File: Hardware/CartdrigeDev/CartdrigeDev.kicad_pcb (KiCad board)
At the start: 2 copper layers, 80 x 14.5 mm, 2 parts, among them J1 Conn_02x30_Odd_Even, J2 PORT1

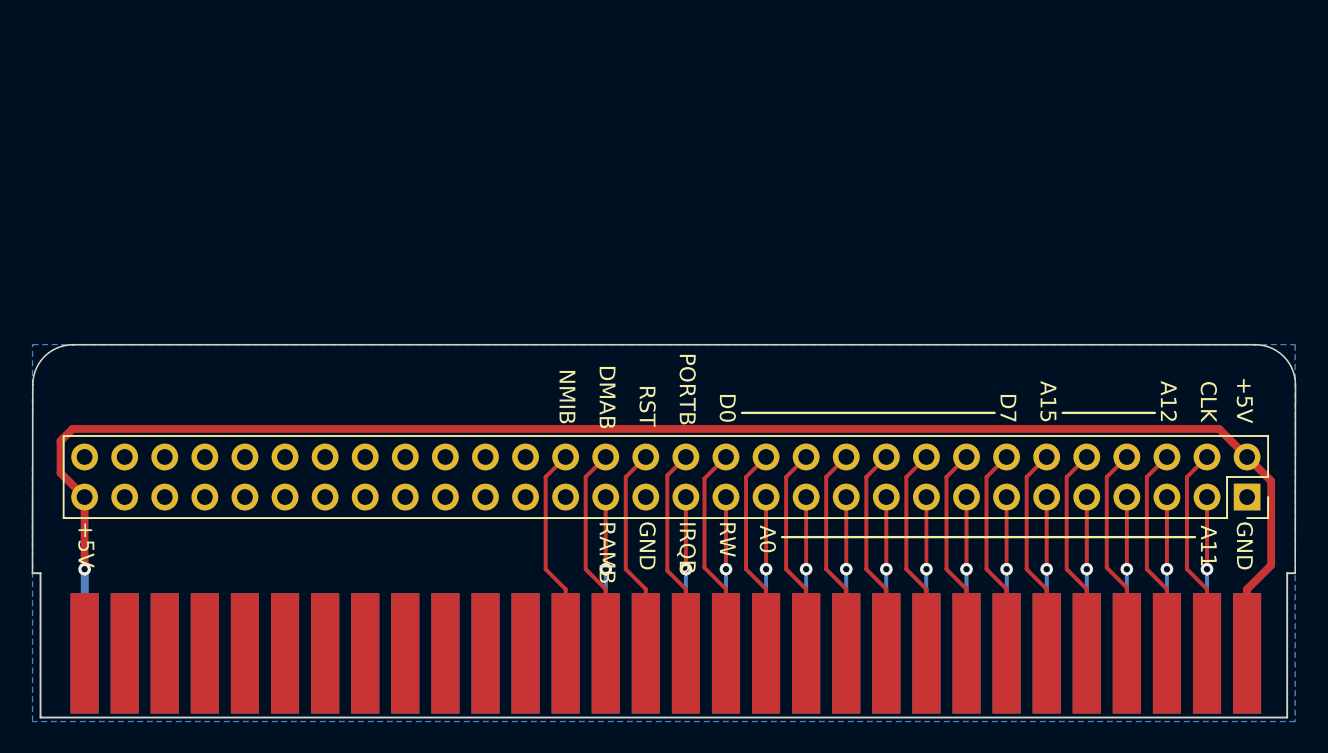
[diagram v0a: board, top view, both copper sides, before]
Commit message: Version 1.3
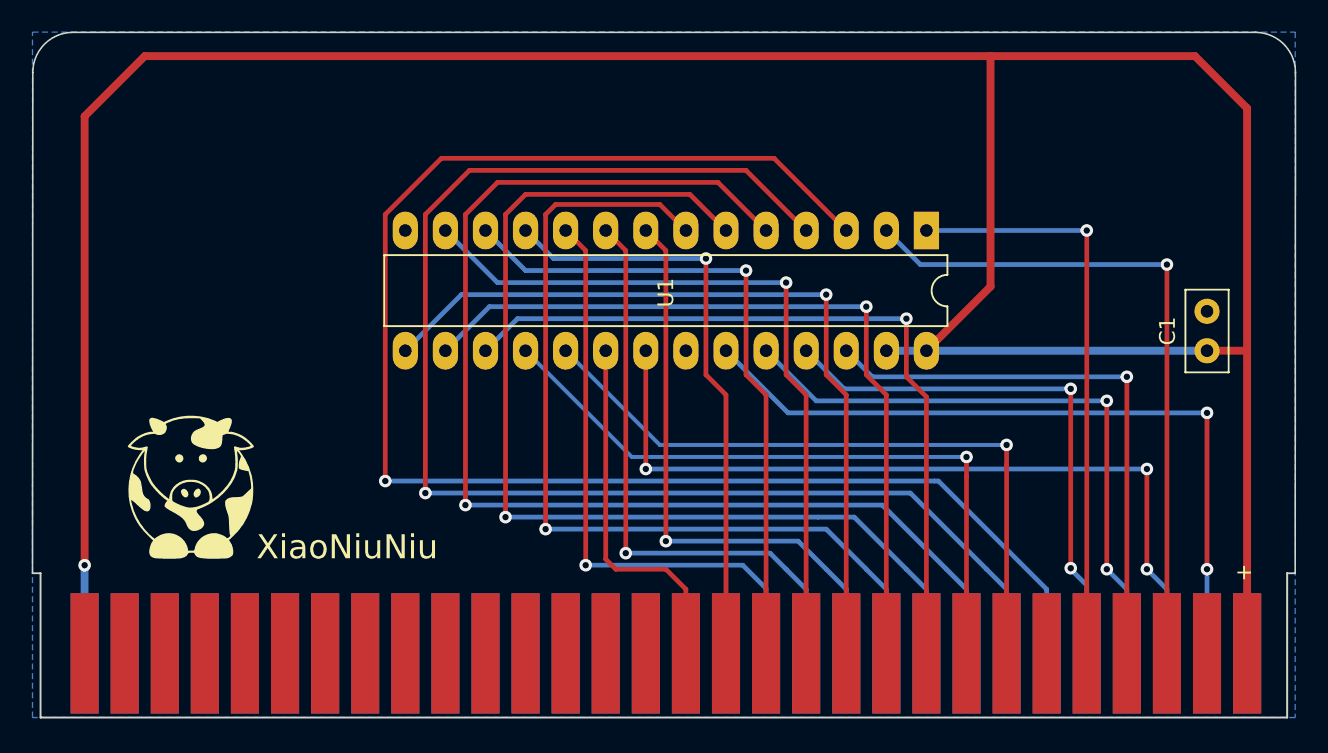
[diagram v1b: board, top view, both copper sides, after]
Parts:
- removed J1: Conn_02x30_Odd_Even, Connector_PinSocket_2.54mm:PinSocket_2x30_P2.54mm_Vertical
- added C1: 100nF, Capacitor_THT:C_Disc_D5.0mm_W2.5mm_P2.50mm, F.Cu at (146.1, 72.5)
- added U1: 28C256, Package_DIP:DIP-28_W7.62mm_LongPads, F.Cu at (128.3, 64.9)
- added XiaoNiuNiu: LOGO, Cow:VerySmallCow, F.Cu at (81.7, 81.2)
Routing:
- net /A7: track 9.91 -> 98.3 mm
- net +5V: track 104.0 -> 188.4 mm
- net /A6: track 9.91 -> 87.9 mm
- net /A5: track 9.91 -> 77.6 mm
- net /A4: track 9.91 -> 67.2 mm
- net /A3: track 9.91 -> 57.0 mm
- net /A10: track 9.91 -> 51.3 mm, vias 1 -> 3
- net /D3: track 13.5 -> 51.4 mm, vias 0 -> 1
- net /A11: track 9.91 -> 47.4 mm, vias 1 -> 2
- net /D4: track 13.5 -> 50.3 mm, vias 0 -> 1
- net /D5: track 13.5 -> 49.2 mm, vias 0 -> 1
- net /D2: track 13.5 -> 47.0 mm, vias 0 -> 1
- net /D7: track 13.5 -> 43.6 mm, vias 0 -> 1
- net /A12: track 13.5 -> 43.3 mm, vias 0 -> 1
- net /D6: track 13.5 -> 43.2 mm, vias 0 -> 1
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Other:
- board size 80 x 14.5 mm -> 80 x 34.3 mm
- board text added: "+"
- board text removed: "+5V"
- board text removed: "A0"
- board text removed: "A11"
- board text removed: "A12"
- board text removed: "A15"
- board text removed: "CLK"
- board text removed: "D0"
- board text removed: "D7"
- board text removed: "DMAB"
- board text removed: "GND"
- board text removed: "IRQB"
- board text removed: "NMIB"
- board text removed: "PORTB"
- board text removed: "RAMB"
- board text removed: "RST"
- board text removed: "RW"
